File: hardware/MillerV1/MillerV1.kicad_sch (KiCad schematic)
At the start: 298 parts, among them Q1 Q12MHz/20pF/10ppm/4P/3.2x2.5mm, U1 CCGM1A1(FBGA-324), U10 RP2040(QFN-56_7x7mm_P0.4mm), U11 TPS62A02ADRLR(SOT-563-6), U12 TPS62A02ADRLR(SOT-563-6), U13 TPS62A02ADRLR(SOT-563-6), U14 TPS62A02ADRLR(SOT-563-6), U15 TPS62A02ADRLR(SOT-563-6), U2 HX7027(SOT-23-3), U3 NA(ZD25WQ16CSIGT(SOIC-8_208mi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, U4 NA(MCP120T-300I/TT(SOT-23-3)), U5 TXB0108PWR(TSSOP-20), U6 TXB0108PWR(TSSOP-20), U7 LY68S3200SLT(SOIC-8_150mil), U8 ZD25WQ16CSIGT(SOIC-8_208mils), U9 LY68S3200SLT(SOIC-8_150mil)

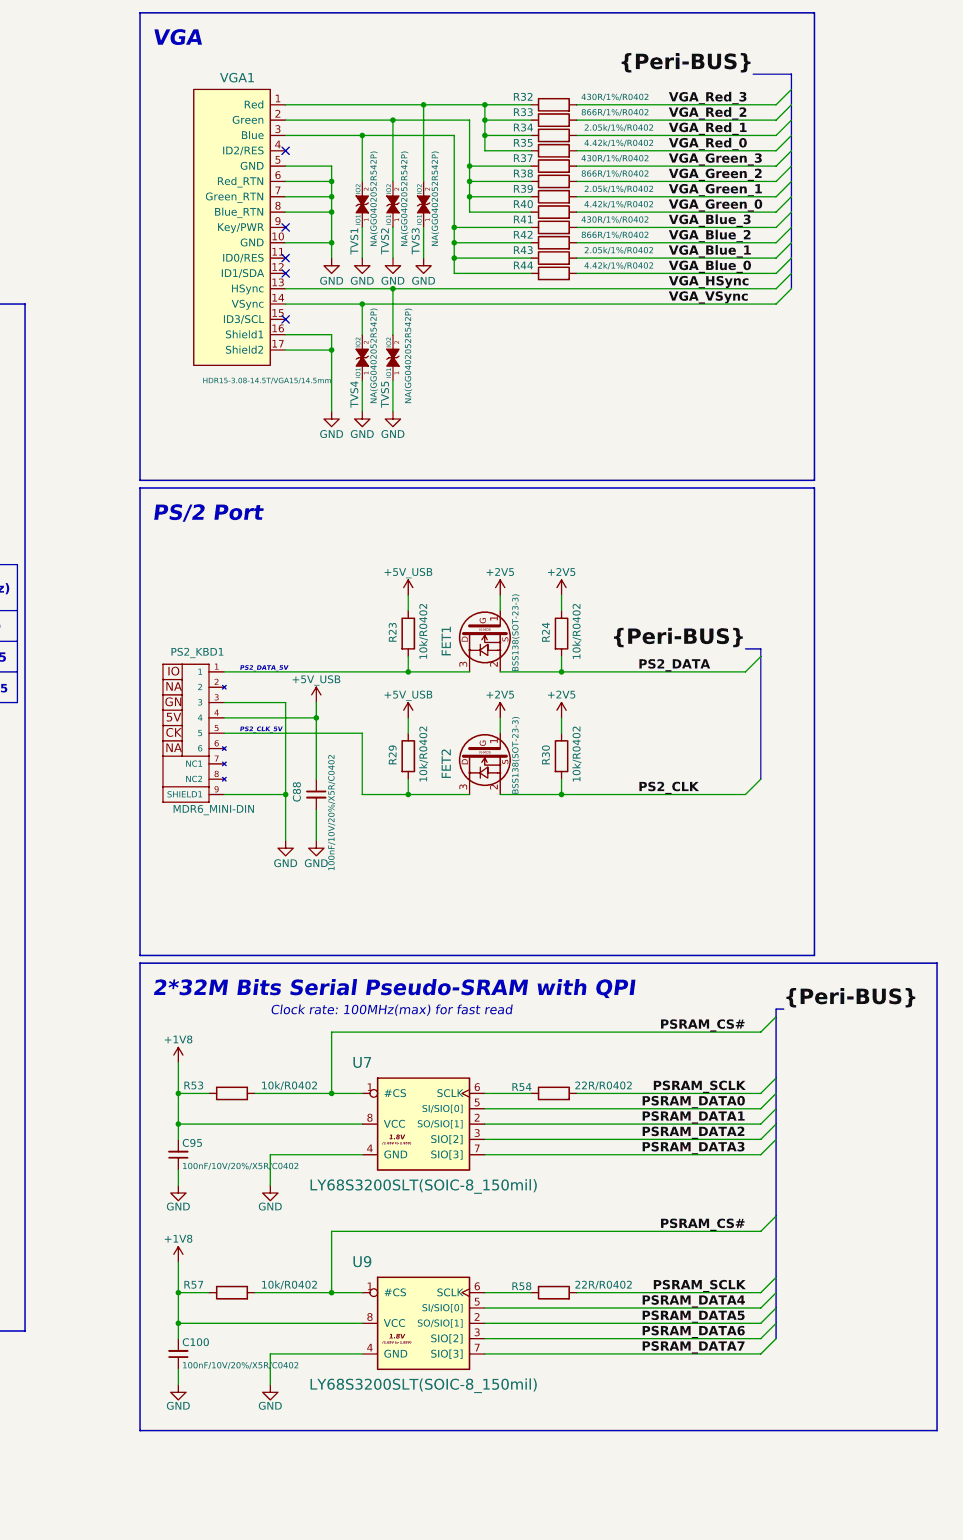
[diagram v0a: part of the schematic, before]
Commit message: updated
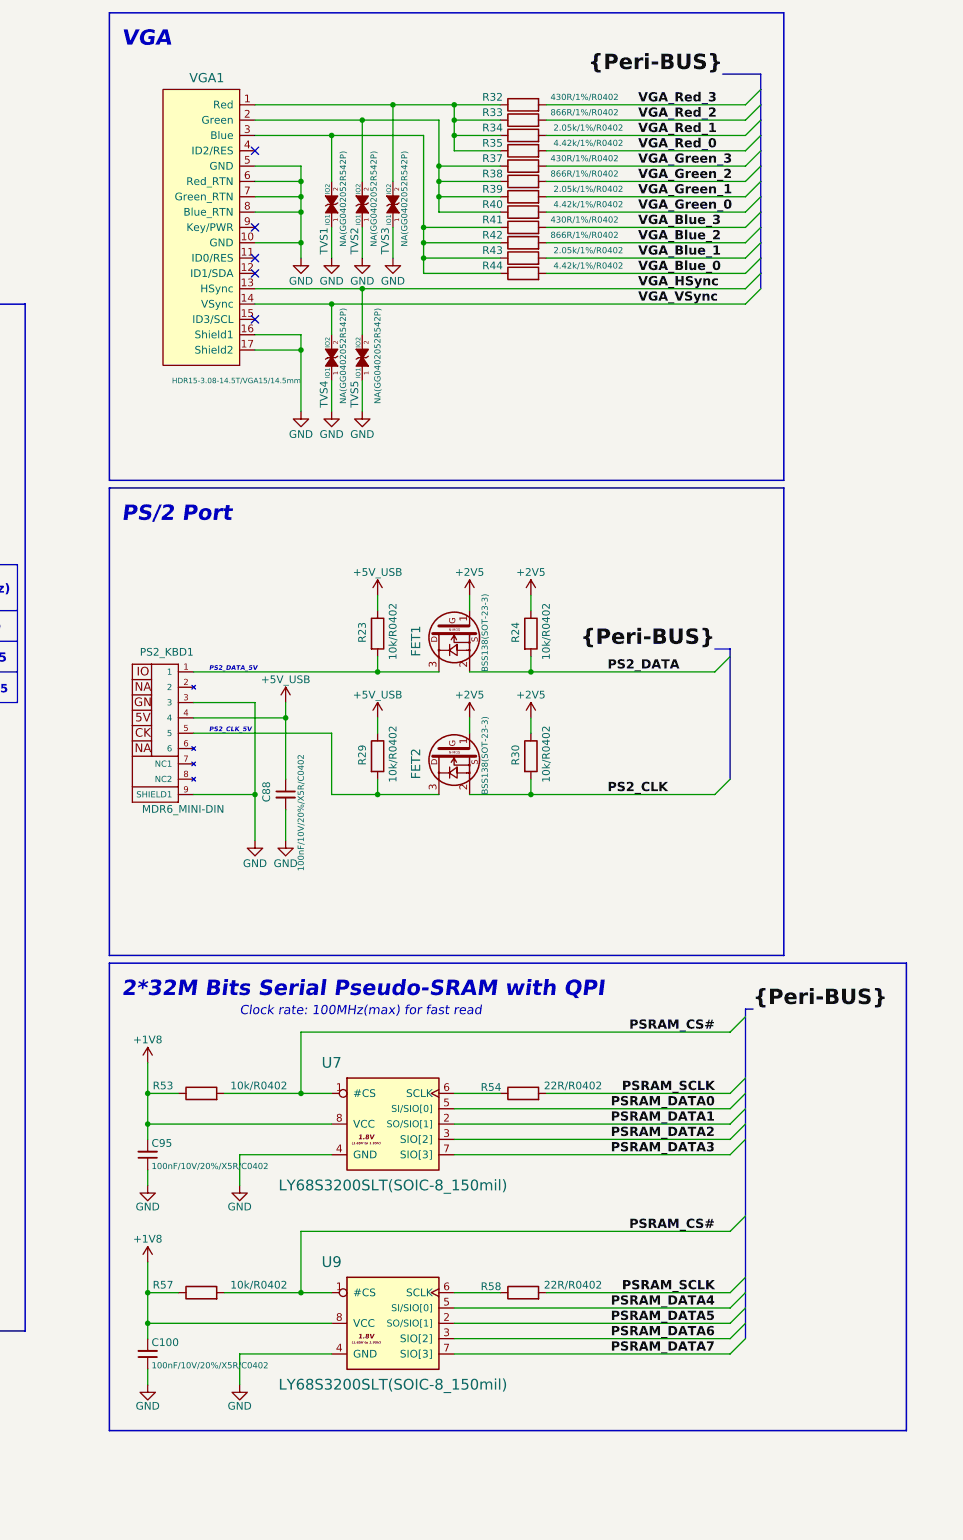
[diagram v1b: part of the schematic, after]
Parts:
- MH1, MH2, MH3, MH4: footprint OLIMEX_Other-FP:Mounting_Hole_Drill-3.3mm_Clerance-7mm -> MountingHole:MountingHole_3.2mm_M3_Pad_Via
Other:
- moved on the sheet: C100, C88, C95, FET1, FET2, PS2_KBD1, R23, R24, R29, R30, R32, R33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

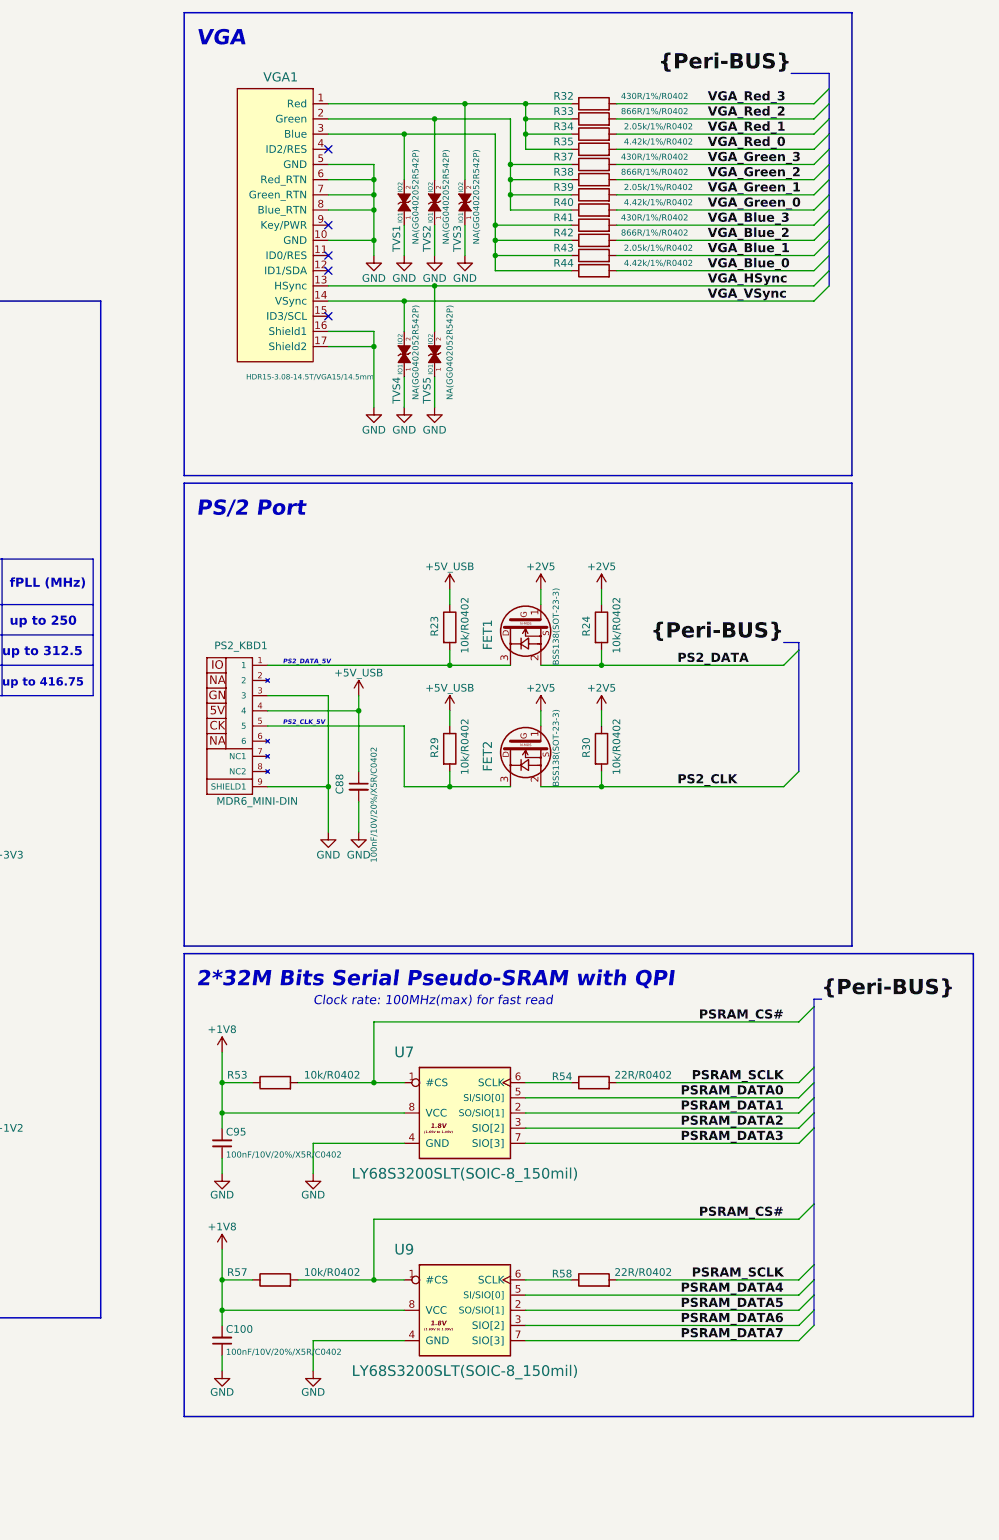
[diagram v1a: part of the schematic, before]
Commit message: made room for tobi
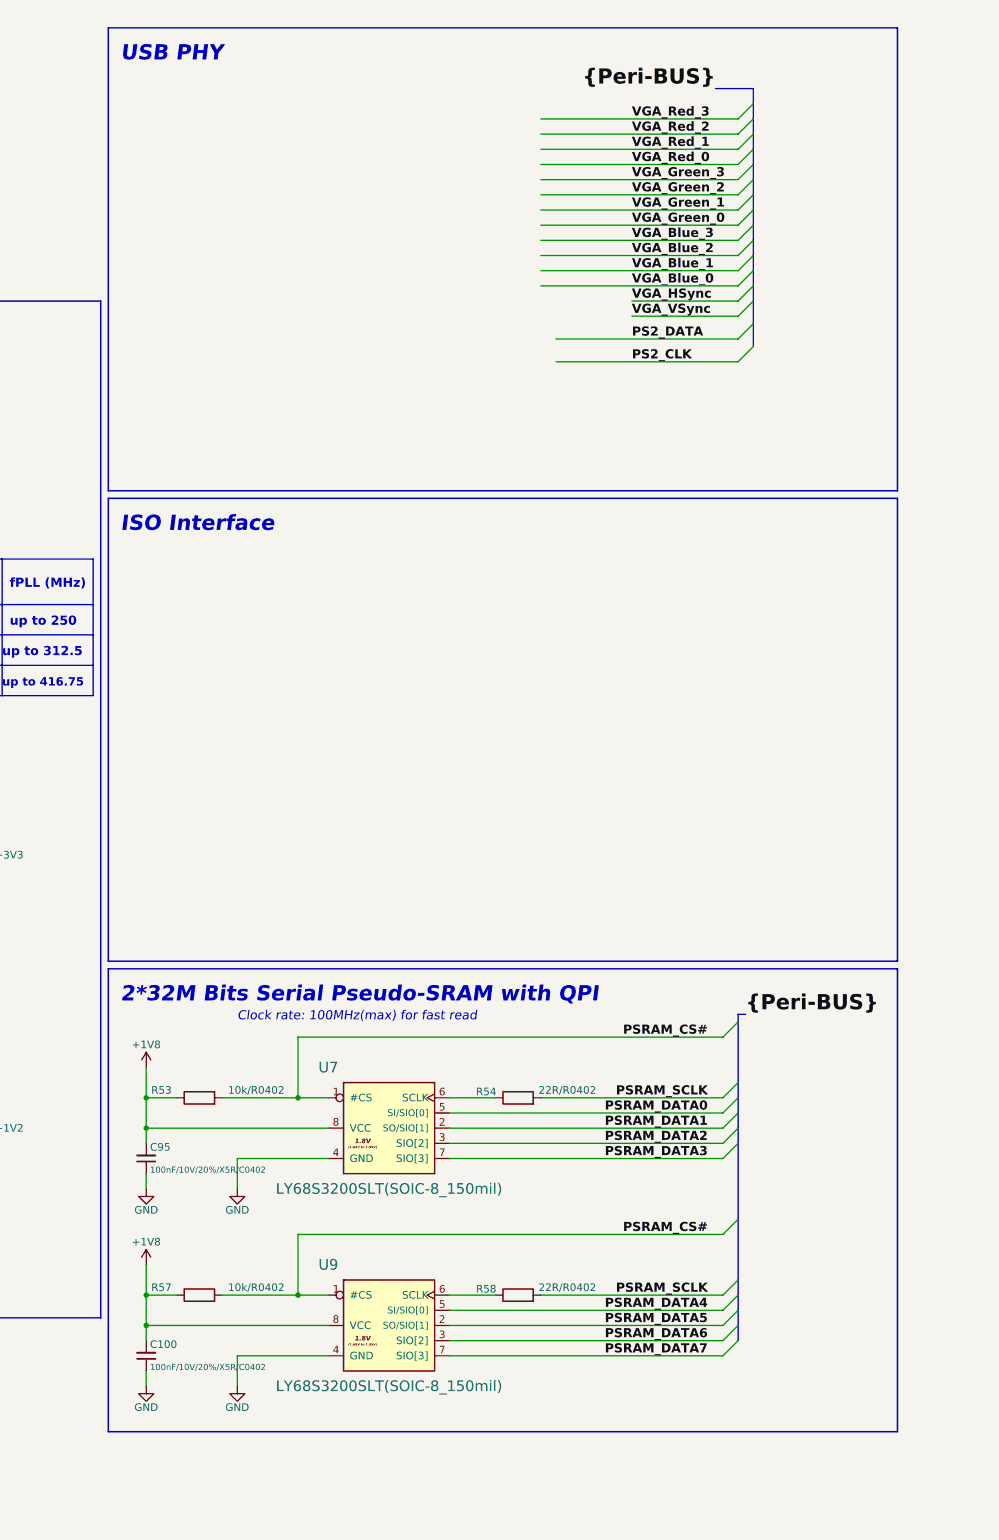
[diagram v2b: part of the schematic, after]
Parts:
- removed C88: 100nF/10V/20%/X5R/C0402, OLIMEX_RLC-FP:C_0402_5MIL_DWS, symbol OLIMEX_RCL:C
- removed FET1, FET2: BSS138(SOT-23-3), OLIMEX_Transistors-FP:SOT23, symbol OLIMEX_Transistors:N-MOS+DIOD
- removed PS2_KBD1: MDR6_MINI-DIN, OLIMEX_Connectors-FP:PS2_MDR6_MINI-DIN, symbol OLIMEX_Connectors:PS2_MDR6_MINI-DIN
- removed R23, R24, R29, R30: 10k/R0402, OLIMEX_RLC-FP:R_0402_5MIL_DWS, symbol OLIMEX_RCL:R
- removed R32, R37, R41: 430R/1%/R0402, OLIMEX_RLC-FP:R_0402_5MIL_DWS, symbol OLIMEX_RCL:R
- removed R33, R38, R42: 866R/1%/R0402, OLIMEX_RLC-FP:R_0402_5MIL_DWS, symbol OLIMEX_RCL:R
- removed R34, R39, R43: 2.05k/1%/R0402, OLIMEX_RLC-FP:R_0402_5MIL_DWS, symbol OLIMEX_RCL:R
- removed R35, R40, R44: 4.42k/1%/R0402, OLIMEX_RLC-FP:R_0402_5MIL_DWS, symbol OLIMEX_RCL:R
- removed TVS1, TVS2, TVS3, TVS4, TVS5: NA(GG0402052R542P), OLIMEX_Diodes-FP:D_0402_5MIL_DWS, symbol OLIMEX_Diodes:GG0402052R542P
- removed VGA1: HDR15-3.08-14.5T/VGA15/14.5mm, OLIMEX_Connectors-FP:VGA15-F(HDR15-3.08-14.5T)_DrillSlot, symbol OLIMEX_Connectors:VGA15-F(CD0515S21J0)
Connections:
- no-connect marks 8 -> 3
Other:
- note added: "ISO Interface"
- note added: "USB PHY"
- note removed: "PS/2 Port"
- note removed: "PS2_CLK_5V"
- note removed: "PS2_DATA_5V"
- note removed: "VGA"
- moved on the sheet: C100, C95, R53, R54, R57, R58, U7, U9
